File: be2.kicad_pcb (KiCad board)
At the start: 2 copper layers, 50 x 30 mm, 31 parts, among them K1 CONN_01X03, K2 CONN_01X02, K3 CONN_01X01, U1 AD620A, U2 TL082, U3 TL082

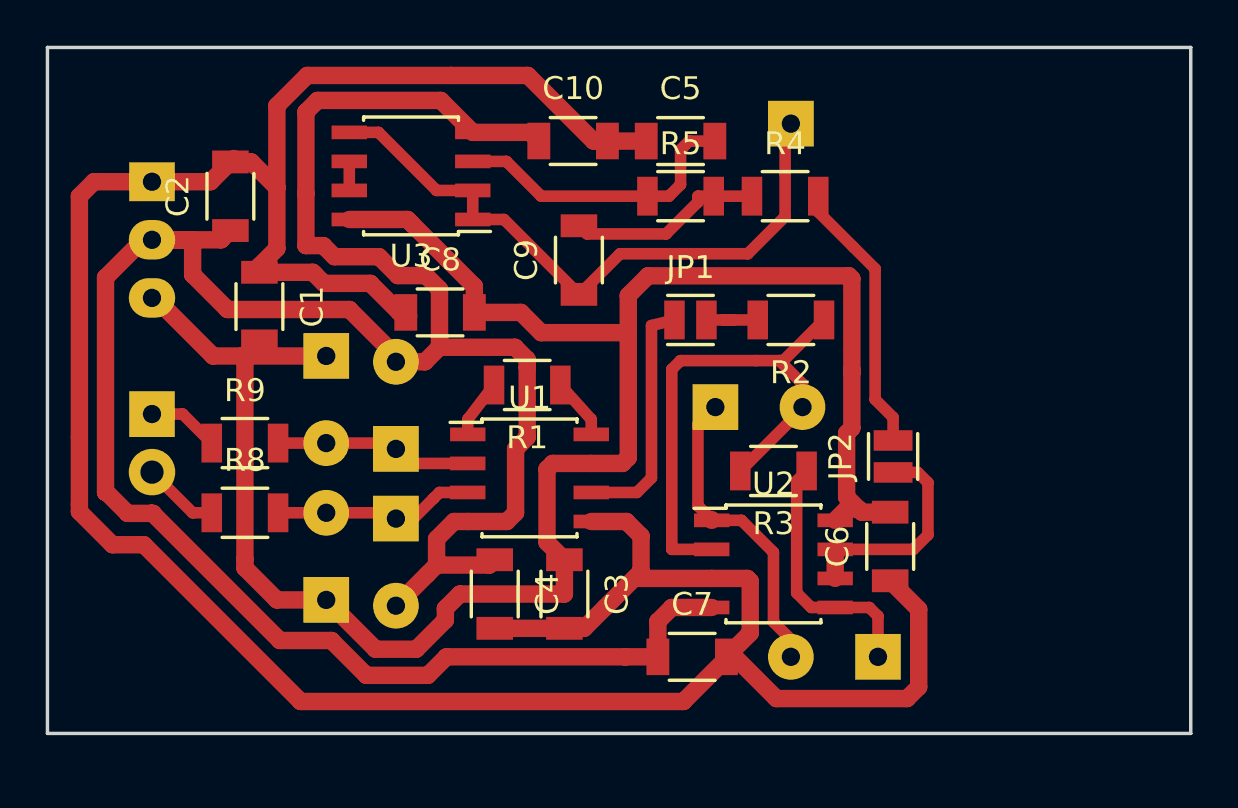
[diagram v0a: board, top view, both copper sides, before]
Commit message: some cleaning on the pcb
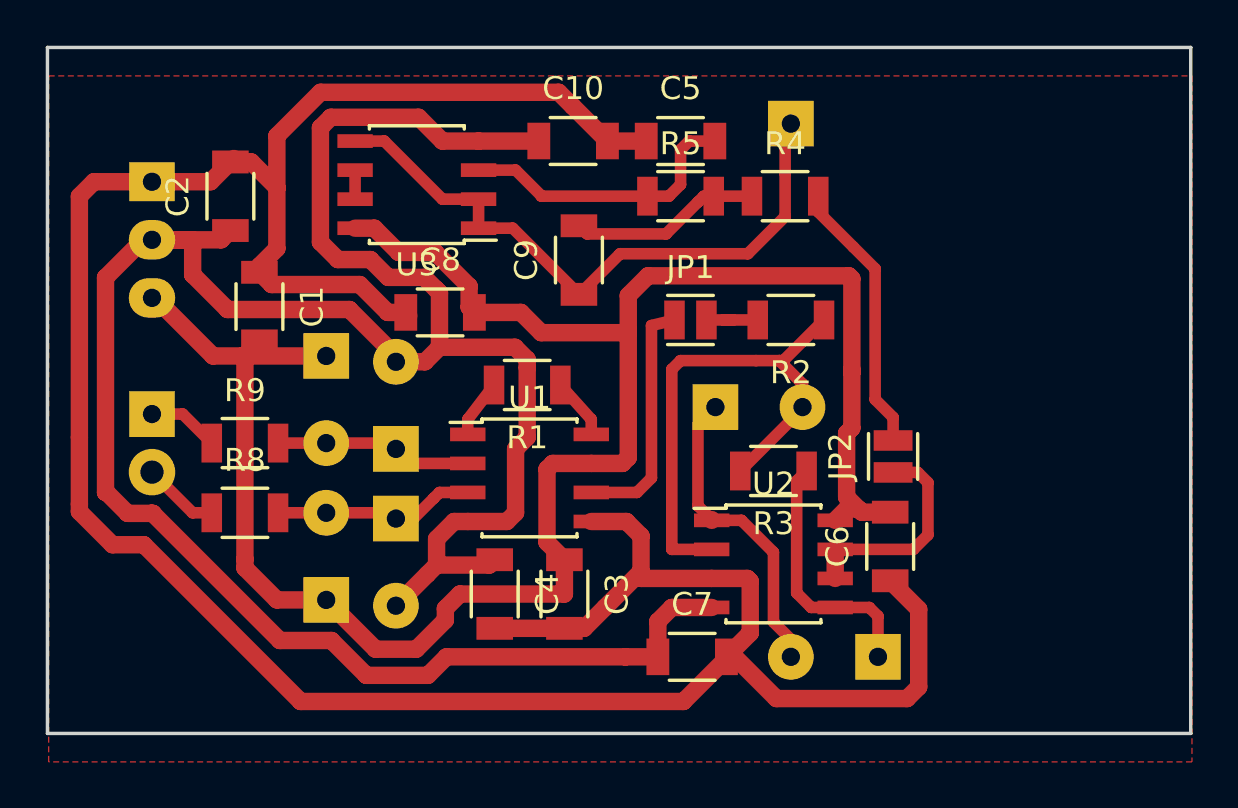
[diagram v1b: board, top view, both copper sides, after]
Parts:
- moved U3 0.46 mm to (28.2, 18.0)
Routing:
- net VSS: track 111.4 -> 109.0 mm
- net GND: track 124.4 -> 123.0 mm
- net VCC: track 91.3 -> 90.7 mm
